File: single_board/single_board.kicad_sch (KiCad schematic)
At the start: 121 parts, among them J1 SWD, J11 SPI Debug, J17 BOOTSEL, J2 USB_C_Receptacle_USB2.0_16P, J3 RST, J30 JST_GH_H, J31 JST_GH_H, J32 PB_Vertical, J33 JST_GH_H, J34 PB_Vertical, J35 JST_GH_H, J36 JST_GH_H, J37 JST_GH_H, J38 PB_Vertical, J39 PB_Vertical, J4 Conn_01x02, J40 PB_Vertical, J41 PB_Vertical, J42 PB_Vertical, J43 PB_Vertical, J44 PB_Vertical, J45 PB_Vertical, J46 PB_Vertical, J47 PB_Vertical, J48 PB_Vertical, J49 PB_Vertical, J5 Conn_01x02, J50 PB_Vertical, J6 Conn_01x02, J7 Conn_01x02, Q1 AO3401A, Q2 AO3401A, Q3 AO3401A, Q4 AO3401A, Q5 2N7002, SW1 Button, U1 AP2112K-3.3, U3 USBLC6-2SC6, U4 LSM6DSV, U5 STM32G474VBTx, Y1 FC-135

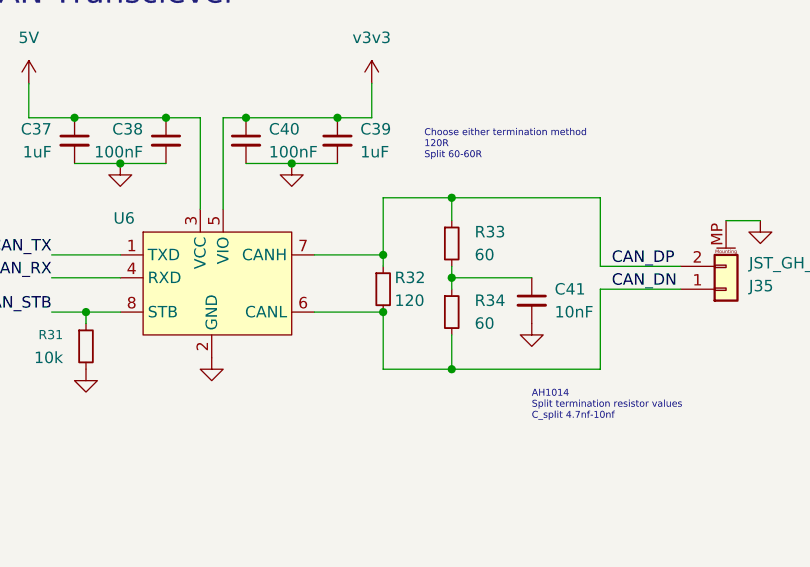
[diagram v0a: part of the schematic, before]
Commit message: PCB Layout
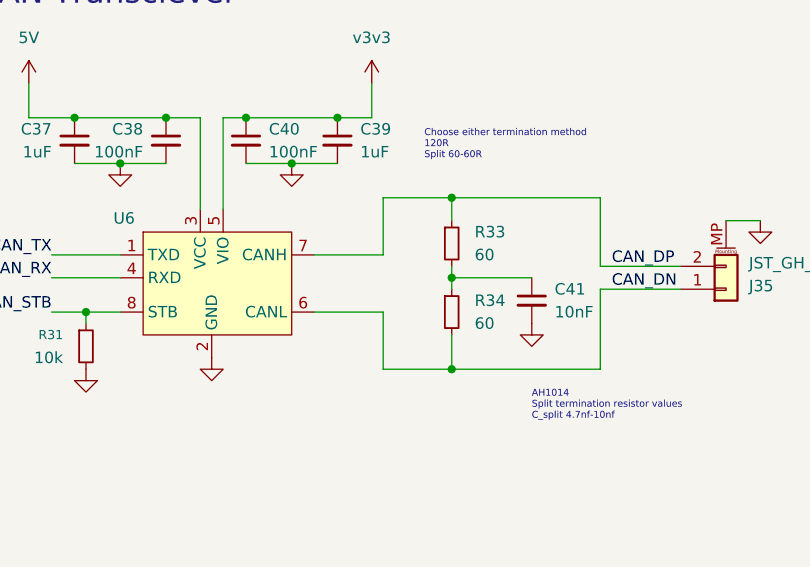
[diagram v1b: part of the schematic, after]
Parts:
- removed R32: 120, Resistor_SMD:R_0402_1005Metric, symbol Device:R_Small
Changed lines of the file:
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@@
 	)
 	(junction
-		(at 261.62 53.34)
-		(diameter 0)
-		(color 0 0 0 0)
-	)
-	(junction
 		(at 38.1 257.81)
 		(diameter 0)
@@
 	)
 	(junction
-		(at 261.62 46.99)
-		(diameter 0)
-		(color 0 0 0 0)
-	)
-	(junction
 		(at 41.91 243.84)
 		(diameter 0)
@@
 	(wire
 		(pts
-			(xy 261.62 46.99) (xy 261.62 48.26)
-		)
-		(stroke
-			(width 0)
-			(type default)
-		)
-	)
-	(wire
-		(pts
 			(xy 294.64 109.22) (xy 297.18 109.22)
 		)
@@
 					(unit 1)
 				)
-			)
-		)
-	)
-	(symbol
-		(lib_id "Device:R_Small")
-		(at 261.62 50.8 0)
-		(unit 1)
-		(body_style 1)
-		(exclude_from_sim no)
-		(in_bom yes)
-		(on_board yes)
-		(in_pos_files yes)
-		(dnp no)
-		(property "Reference" "R32"
-			(at 262.89 49.5299 0)
-			(show_name no)
-			(do_not_autoplace no)
-			(effects
-				(font
-					(size 1.27 1.27)
-				)
-				(justify left)
-			)
-		)
-		(property "Value" "120"
-			(at 262.89 52.0699 0)
-			(show_name no)
-			(do_not_autoplace no)
-			(effects
-				(font
-					(size 1.27 1.27)
-				)
-				(justify left)
-			)
-		)
-		(property "Footprint" "Resistor_SMD:R_0402_1005Metric"
-			(at 261.62 50.8 0)
-			(hide yes)
-			(show_name no)
-			(do_not_autoplace no)
-			(effects
-				(font
-					(size 1.27 1.27)
-				)
-			)
-		)
-		(property "Datasheet" ""
-			(at 261.62 50.8 0)
-			(hide yes)
-			(show_name no)
-			(do_not_autoplace no)
-			(effects
-				(font
-					(size 1.27 1.27)
-				)
-			)
-		)
-		(property "Description" "Resistor, small symbol"
-			(at 261.62 50.8 0)
-			(hide yes)
-			(show_name no)
-			(do_not_autoplace no)
-			(effects
-				(font
-					(size 1.27 1.27)
-				)
-			)
-		)
-		(pin "1"
-		)
-		(pin "2"
-		)
-		(instances
-			(project "single_board"
-				(path "/ae10586e-ebf8-402d-a979-c2f011cdeee2"
-					(reference "R32")
-					(unit 1)
-				)
